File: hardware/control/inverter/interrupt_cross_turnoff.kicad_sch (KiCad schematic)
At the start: 16 parts, among them SW1 SW_DPDT_x2, SW2 SW_DPDT_x2, U13 74HC08, U14 74HC74, U16 74HC14, U17 74HC08, U18 74HC14, U19 74HC14, U20 74HC08

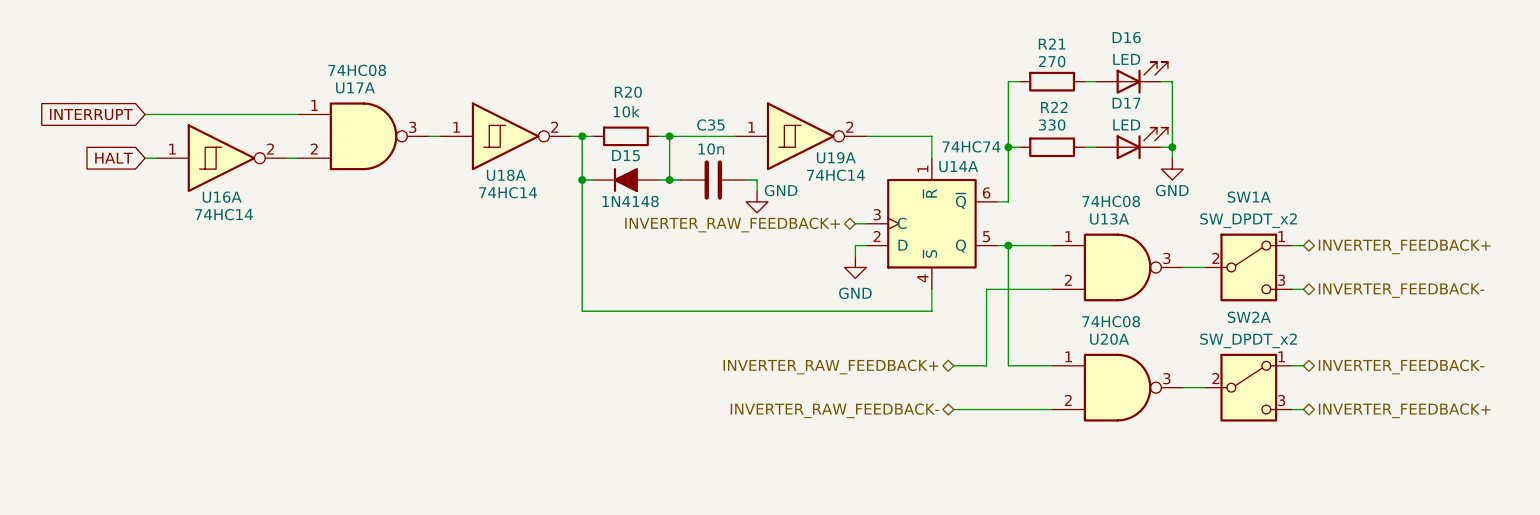
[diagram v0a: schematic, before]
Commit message: update
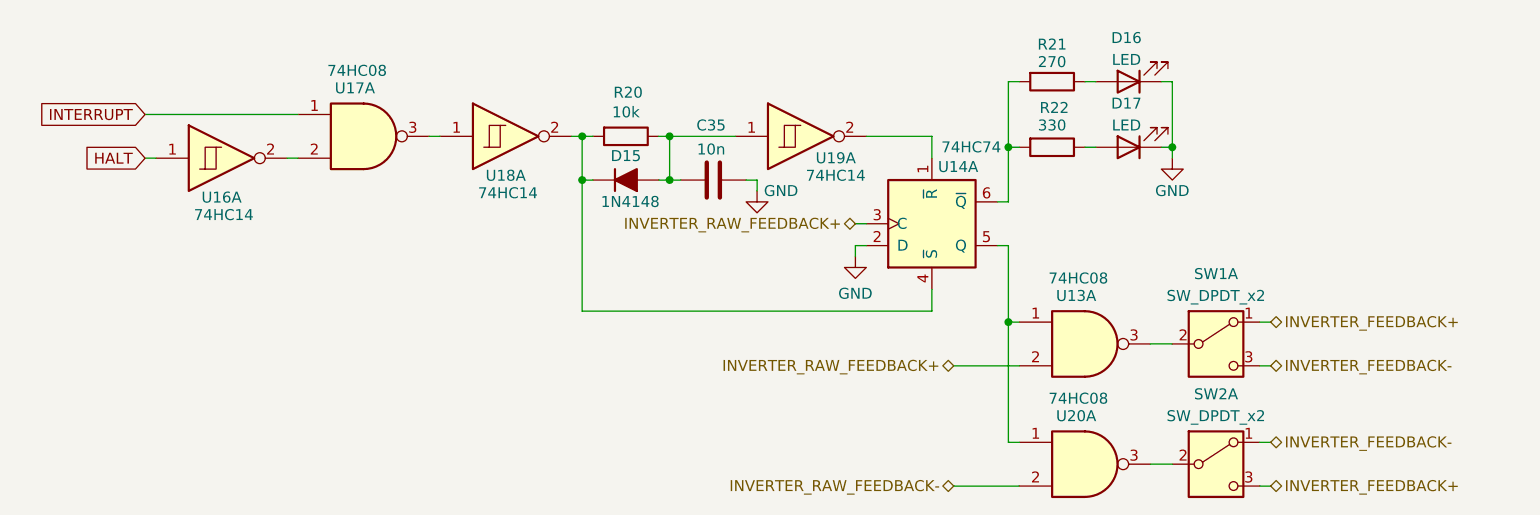
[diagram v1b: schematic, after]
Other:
- moved on the sheet: SW1A, SW2A, U13A, U20A
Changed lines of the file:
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@@
 	)
 	(junction
-		(at 167.64 102.87)
+		(at 167.64 111.76)
 		(diameter 0)
 		(color 0 0 0 0)
@@
 	(wire
 		(pts
-			(xy 167.64 102.87) (xy 167.64 116.84)
+			(xy 167.64 111.76) (xy 167.64 125.73)
 		)
 		(stroke
@@
 	(wire
 		(pts
+			(xy 167.64 102.87) (xy 166.37 102.87)
+		)
+		(stroke
+			(width 0)
+			(type default)
+		)
+	)
+	(wire
+		(pts
 			(xy 100.33 90.17) (xy 101.6 90.17)
 		)
@@
 	(wire
 		(pts
-			(xy 165.1 107.95) (xy 172.72 107.95)
-		)
-		(stroke
-			(width 0)
-			(type default)
-		)
-	)
-	(wire
-		(pts
 			(xy 118.11 90.17) (xy 119.38 90.17)
 		)
@@
 	(wire
 		(pts
-			(xy 166.37 102.87) (xy 167.64 102.87)
-		)
-		(stroke
-			(width 0)
-			(type default)
-		)
-	)
-	(wire
-		(pts
 			(xy 185.42 91.44) (xy 186.69 91.44)
 		)
@@
 	(wire
 		(pts
-			(xy 187.96 119.38) (xy 190.5 119.38)
+			(xy 184.15 128.27) (xy 186.69 128.27)
 		)
 		(stroke
@@
 	(wire
 		(pts
-			(xy 161.29 116.84) (xy 165.1 116.84)
+			(xy 161.29 116.84) (xy 168.91 116.84)
 		)
 		(stroke
@@
 	(wire
 		(pts
-			(xy 167.64 102.87) (xy 172.72 102.87)
+			(xy 167.64 111.76) (xy 168.91 111.76)
 		)
 		(stroke
@@
 	(wire
 		(pts
-			(xy 165.1 116.84) (xy 165.1 107.95)
-		)
-		(stroke
-			(width 0)
-			(type default)
-		)
-	)
-	(wire
-		(pts
 			(xy 138.43 95.25) (xy 138.43 96.52)
 		)
@@
 	(wire
 		(pts
-			(xy 167.64 116.84) (xy 172.72 116.84)
-		)
-		(stroke
-			(width 0)
-			(type default)
-		)
-	)
-	(wire
-		(pts
-			(xy 200.66 107.95) (xy 201.93 107.95)
-		)
-		(stroke
-			(width 0)
-			(type default)
-		)
-	)
-	(wire
-		(pts
-			(xy 200.66 121.92) (xy 201.93 121.92)
+			(xy 167.64 125.73) (xy 168.91 125.73)
+		)
+		(stroke
+			(width 0)
+			(type default)
+		)
+	)
+	(wire
+		(pts
+			(xy 196.85 116.84) (xy 198.12 116.84)
+		)
+		(stroke
+			(width 0)
+			(type default)
+		)
+	)
+	(wire
+		(pts
+			(xy 196.85 130.81) (xy 198.12 130.81)
 		)
 		(stroke
@@
 	(wire
 		(pts
-			(xy 200.66 102.87) (xy 201.93 102.87)
-		)
-		(stroke
-			(width 0)
-			(type default)
-		)
-	)
-	(wire
-		(pts
-			(xy 161.29 121.92) (xy 172.72 121.92)
+			(xy 167.64 111.76) (xy 167.64 102.87)
+		)
+		(stroke
+			(width 0)
+			(type default)
+		)
+	)
+	(wire
+		(pts
+			(xy 196.85 111.76) (xy 198.12 111.76)
+		)
+		(stroke
+			(width 0)
+			(type default)
+		)
+	)
+	(wire
+		(pts
+			(xy 161.29 130.81) (xy 168.91 130.81)
 		)
 		(stroke
@@
 	(wire
 		(pts
-			(xy 200.66 116.84) (xy 201.93 116.84)
-		)
-		(stroke
-			(width 0)
-			(type default)
-		)
-	)
-	(wire
-		(pts
-			(xy 187.96 105.41) (xy 190.5 105.41)
+			(xy 196.85 125.73) (xy 198.12 125.73)
+		)
+		(stroke
+			(width 0)
+			(type default)
+		)
+	)
+	(wire
+		(pts
+			(xy 184.15 114.3) (xy 186.69 114.3)
 		)
 		(stroke
@@
 	(hierarchical_label "INVERTER_RAW_FEEDBACK-"
 		(shape bidirectional)
-		(at 161.29 121.92 180)
+		(at 161.29 130.81 180)
 		(effects
 			(font
@@
 	(hierarchical_label "INVERTER_FEEDBACK+"
 		(shape bidirectional)
-		(at 201.93 102.87 0)
+		(at 198.12 111.76 0)
 		(effects
 			(font
@@
 	(hierarchical_label "INVERTER_FEEDBACK-"
 		(shape bidirectional)
-		(at 201.93 107.95 0)
+		(at 198.12 116.84 0)
 		(effects
 			(font
@@
 	(hierarchical_label "INVERTER_FEEDBACK+"
 		(shape bidirectional)
-		(at 201.93 121.92 0)
+		(at 198.12 130.81 0)
 		(effects
 			(font
@@
 	(hierarchical_label "INVERTER_FEEDBACK-"
 		(shape bidirectional)
-		(at 201.93 116.84 0)
+		(at 198.12 125.73 0)
 		(effects
 			(font
@@
 	(symbol
 		(lib_id "74xx:74HC00")
-		(at 180.34 119.38 0)
+		(at 176.53 128.27 0)
 		(unit 1)
 		(exclude_from_sim no)
@@
 		(dnp no)
 		(property "Reference" "U20"
-			(at 179.324 113.792 0)
+			(at 175.514 122.682 0)
 			(effects
 				(font
@@
 		)
 		(property "Value" "74HC08"
-			(at 179.578 111.76 0)
+			(at 175.768 120.65 0)
 			(effects
 				(font
@@
 		)
 		(property "Footprint" ""
-			(at 180.34 119.38 0)
+			(at 176.53 128.27 0)
 			(effects
 				(font
@@
 		)
 		(property "Datasheet" "http://www.ti.com/lit/gpn/sn74hc00"
-			(at 180.34 119.38 0)
+			(at 176.53 128.27 0)
 			(effects
 				(font
@@
 		)
 		(property "Description" "quad 2-input NAND gate"
-			(at 180.34 119.38 0)
+			(at 176.53 128.27 0)
 			(effects
 				(font
@@
 	(symbol
 		(lib_id "Switch:SW_DPDT_x2")
-		(at 195.58 119.38 0)
+		(at 191.77 128.27 0)
 		(unit 1)
 		(exclude_from_sim no)
@@
 		(dnp no)
 		(property "Reference" "SW2"
-			(at 195.58 111.252 0)
+			(at 191.77 120.142 0)
 			(effects
 				(font
@@
 		)
 		(property "Value" "SW_DPDT_x2"
-			(at 195.58 113.792 0)
+			(at 191.77 122.682 0)
 			(effects
 				(font
@@
 		)
 		(property "Footprint" ""
-			(at 195.58 119.38 0)
+			(at 191.77 128.27 0)
 			(effects
 				(font
@@
 		)
 		(property "Datasheet" "~"
-			(at 195.58 119.38 0)
+			(at 191.77 128.27 0)
 			(effects
 				(font
@@
 		)
 		(property "Description" "Switch, dual pole double throw, separate symbols"
-			(at 195.58 119.38 0)
+			(at 191.77 128.27 0)
 			(effects
 				(font
@@
 	(symbol
 		(lib_id "74xx:74HC00")
-		(at 180.34 105.41 0)
+		(at 176.53 114.3 0)
 		(unit 1)
 		(exclude_from_sim no)
@@
 		(dnp no)
 		(property "Reference" "U13"
-			(at 179.324 99.822 0)
+			(at 175.514 108.712 0)
 			(effects
 				(font
@@
 		)
 		(property "Value" "74HC08"
-			(at 179.578 97.79 0)
+			(at 175.768 106.68 0)
 			(effects
 				(font
@@
 		)
 		(property "Footprint" ""
-			(at 180.34 105.41 0)
+			(at 176.53 114.3 0)
 			(effects
 				(font
@@
 		)
 		(property "Datasheet" "http://www.ti.com/lit/gpn/sn74hc00"
-			(at 180.34 105.41 0)
+			(at 176.53 114.3 0)
 			(effects
 				(font
@@
 		)
 		(property "Description" "quad 2-input NAND gate"
-			(at 180.34 105.41 0)
+			(at 176.53 114.3 0)
 			(effects
 				(font
@@
 	(symbol
 		(lib_id "Switch:SW_DPDT_x2")
-		(at 195.58 105.41 0)
+		(at 191.77 114.3 0)
 		(unit 1)
 		(exclude_from_sim no)
@@
 		(dnp no)
 		(property "Reference" "SW1"
-			(at 195.58 97.282 0)
+			(at 191.77 106.172 0)
 			(effects
 				(font
@@
 		)
 		(property "Value" "SW_DPDT_x2"
-			(at 195.58 99.822 0)
+			(at 191.77 108.712 0)
 			(effects
 				(font
@@
 		)
 		(property "Footprint" ""
-			(at 195.58 105.41 0)
+			(at 191.77 114.3 0)
 			(effects
 				(font
@@
 		)
 		(property "Datasheet" "~"
-			(at 195.58 105.41 0)
+			(at 191.77 114.3 0)
 			(effects
 				(font
@@
 		)
 		(property "Description" "Switch, dual pole double throw, separate symbols"
-			(at 195.58 105.41 0)
-			(effects
-				(font
+			(at 191.77 114.3 0)
+			(effects
+				(font

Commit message: update right about freaking everything
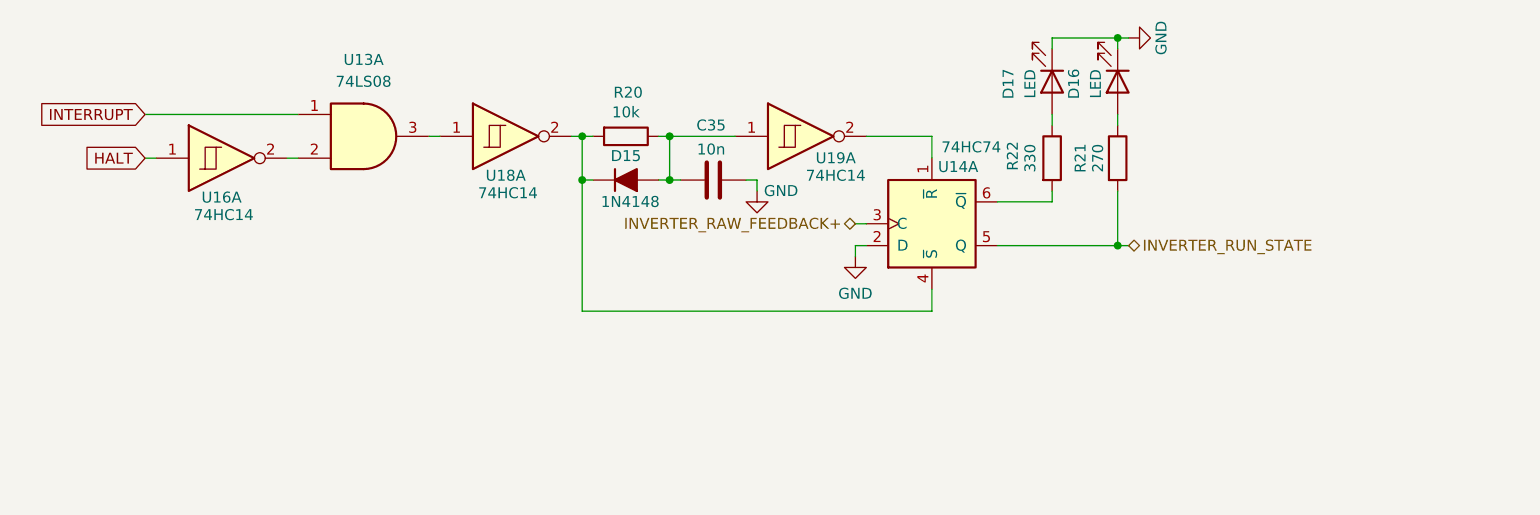
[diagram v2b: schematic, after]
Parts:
- removed SW1, SW2: SW_DPDT_x2, symbol Switch:SW_DPDT_x2
- removed U13, U17, U20: 74HC08, symbol 74xx:74HC00
- added U13: 74LS08, symbol 74xx:74LS08
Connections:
- net INTERRUPT: now also U13.1
- net INVERTER_RUN_STATE: now reaches U14.5 (Q)
- net INVERTER_RUN_STATE: now also R21.2
- net at R22.2, U14.6 (~{Q}): no longer R21.2
- net at U16.2: now also U13.2
- net at U18.1: now also U13.3
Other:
- moved on the sheet: D16, D17, R21, R22
